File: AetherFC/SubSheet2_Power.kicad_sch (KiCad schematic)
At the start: 32 parts, among them U4 MIC5219-3.3YM5, U8 MP9943GQ-Z, U9 MP9943GQ-Z

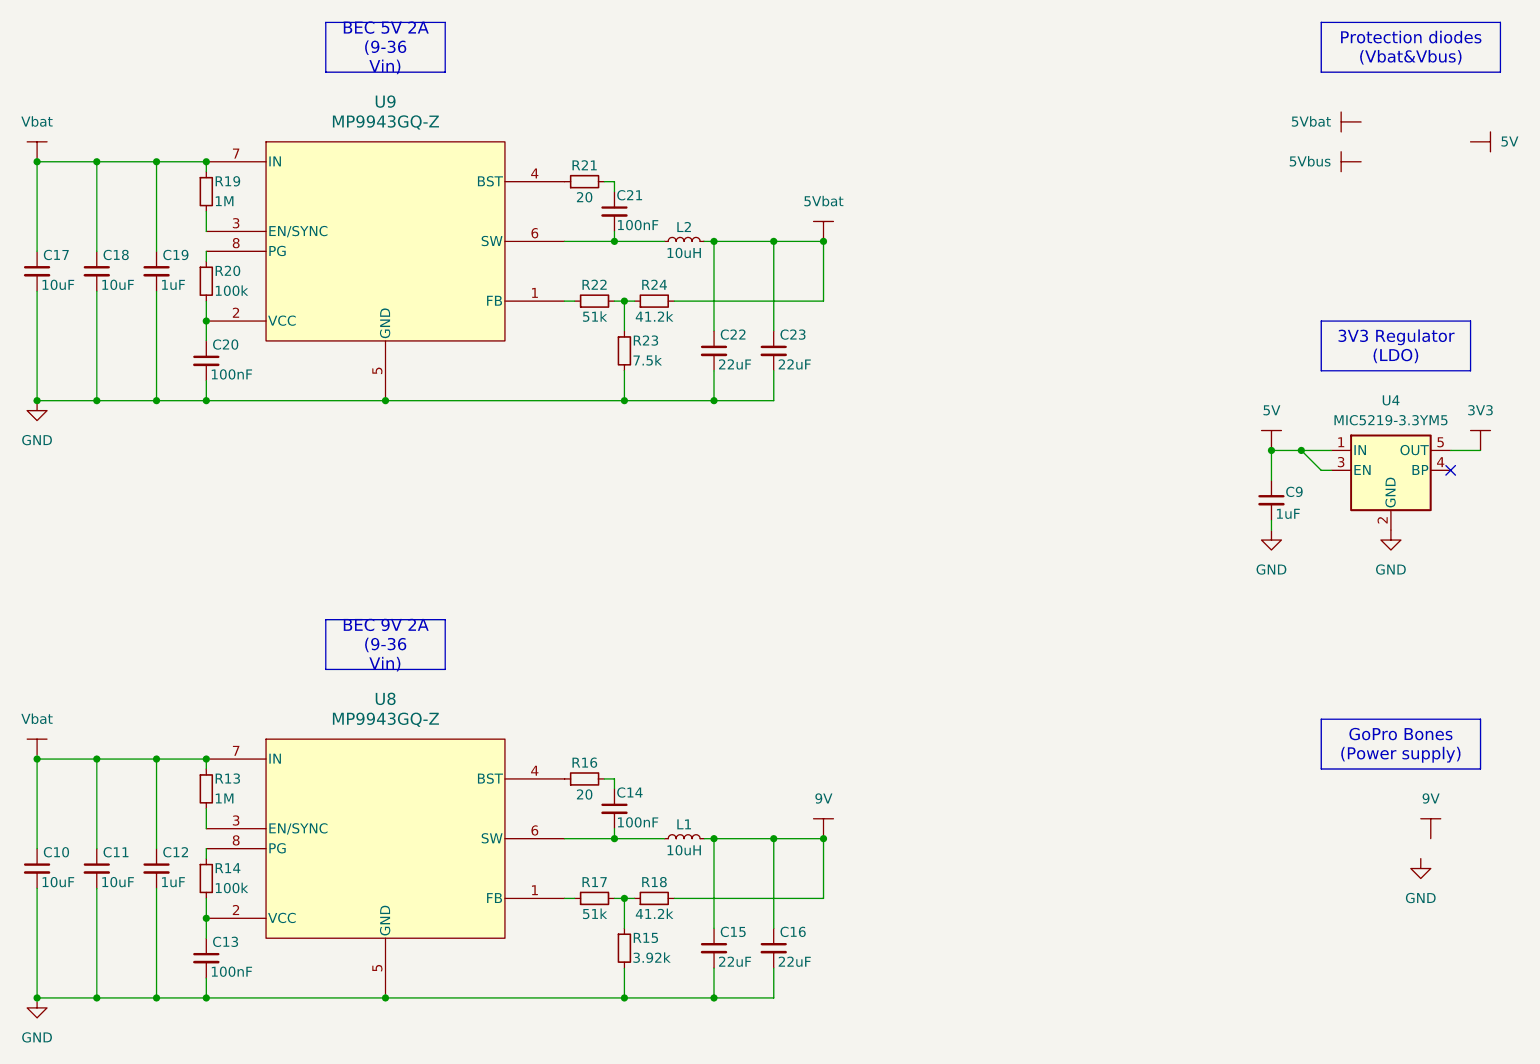
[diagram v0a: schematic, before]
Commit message: Repo cleaned up before ESC schematics
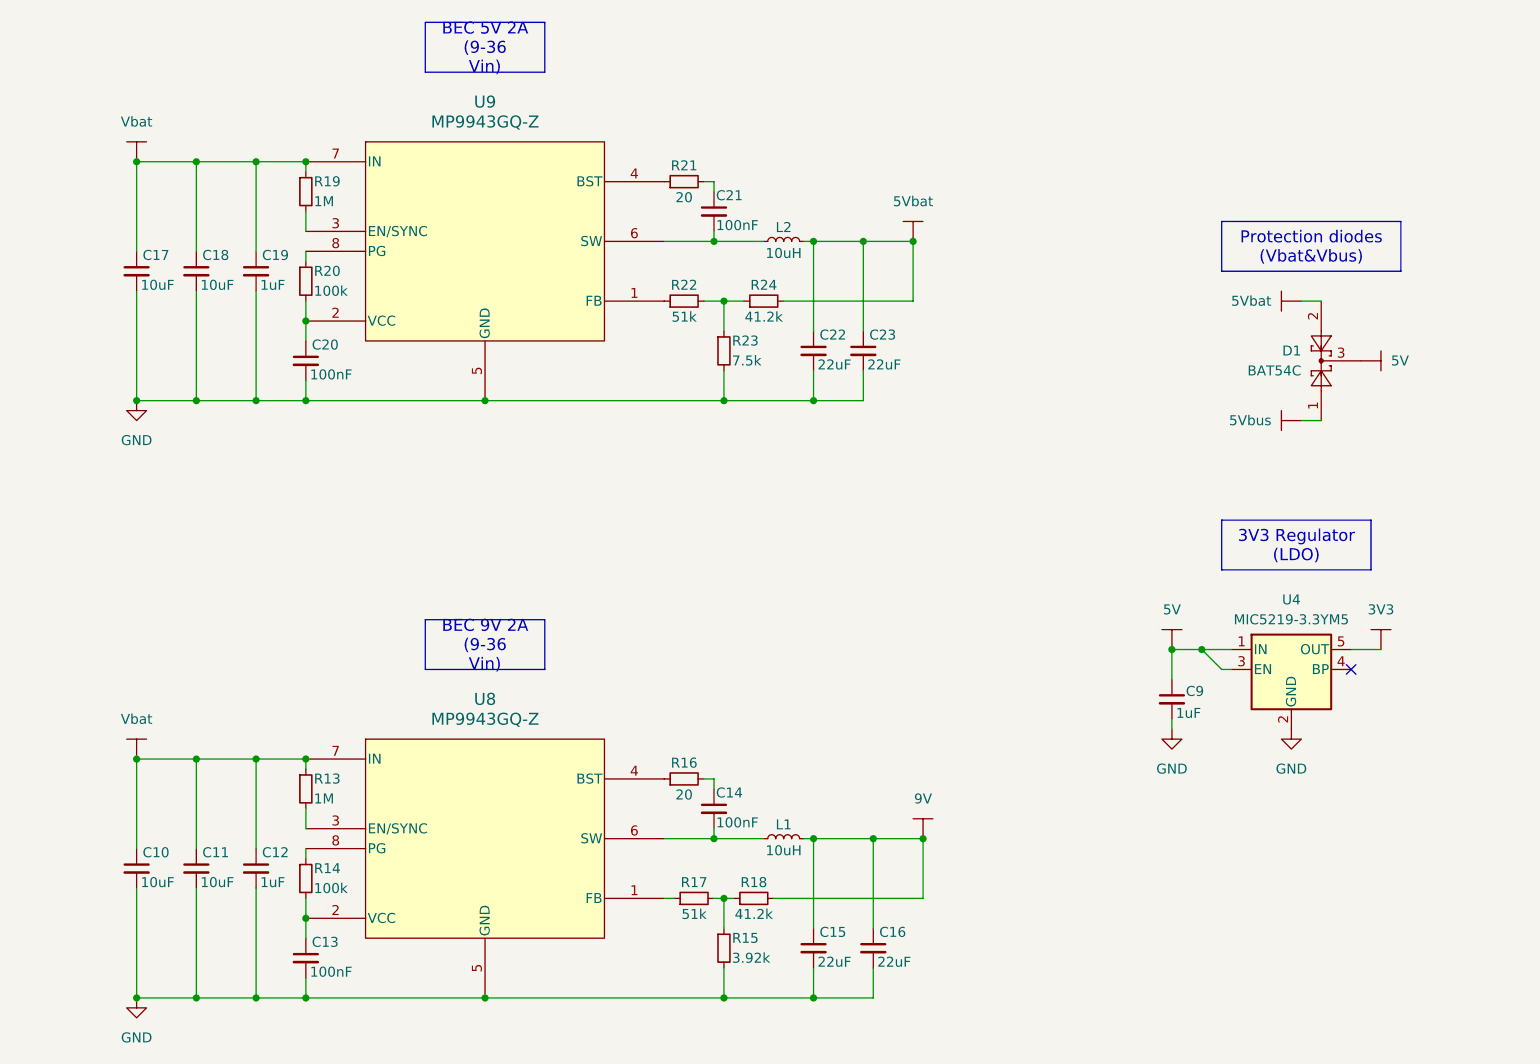
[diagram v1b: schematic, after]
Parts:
- added D1: BAT54C, Package_TO_SOT_SMD:SOT-23, symbol Diode:BAT54C
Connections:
- net 5V: now also D1.3
- net 5Vbat: now also D1.2
- net 5Vbus: now also D1.1
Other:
- company: (none) -> https://github.com/Lpwlk/AetherStack
- moved on the sheet: C10, C11, C12, C13, C14, C15, C16, C17, C18, C19, C20, C21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
